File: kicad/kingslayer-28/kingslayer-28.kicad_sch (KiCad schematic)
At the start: 68 parts, among them IC1 STM32F303CCT7, IC2 IS31FL3731-QFLS2-TR, K1 KEYSW, K10 KEYSW, K11 KEYSW, K12 KEYSW, K13 KEYSW, K14 KEYSW, K15 KEYSW, K16 KEYSW, K17 KEYSW, K18 KEYSW, K19 KEYSW, K2 KEYSW, K20 KEYSW, K21 KEYSW, K22 KEYSW, K23 KEYSW, K24 KEYSW, K25 KEYSW, K26 KEYSW, K27 KEYSW, K28 KEYSW, K3 KEYSW, K4 KEYSW, K5 KEYSW, K6 KEYSW, K7 KEYSW, K8 KEYSW, K9 KEYSW, SW1 SW_PUSH, X1 XTAL_GND

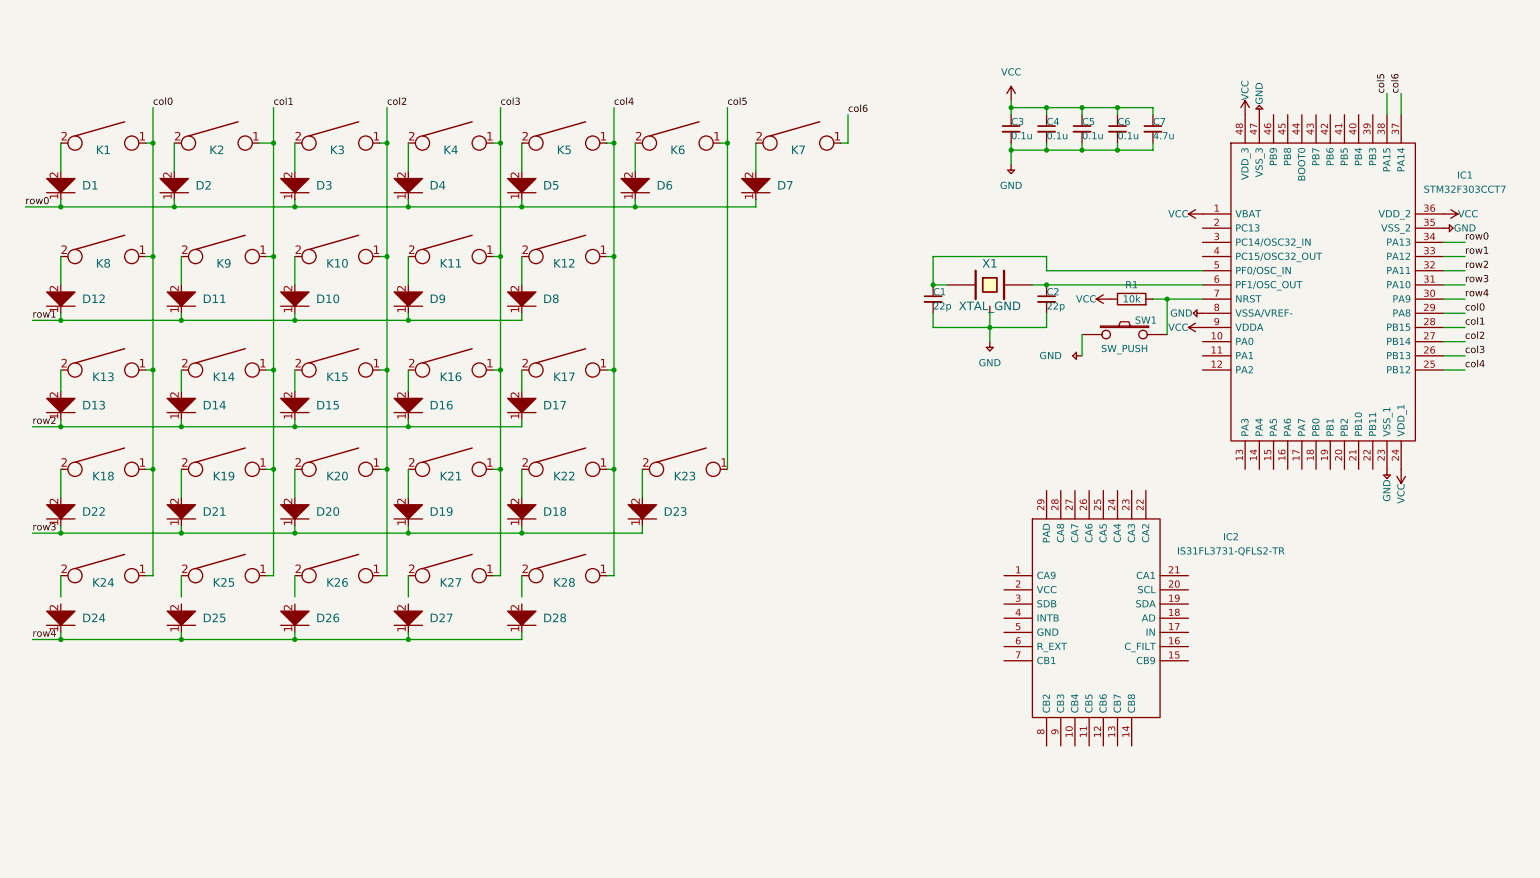
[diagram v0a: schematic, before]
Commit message: tidy up the schematic
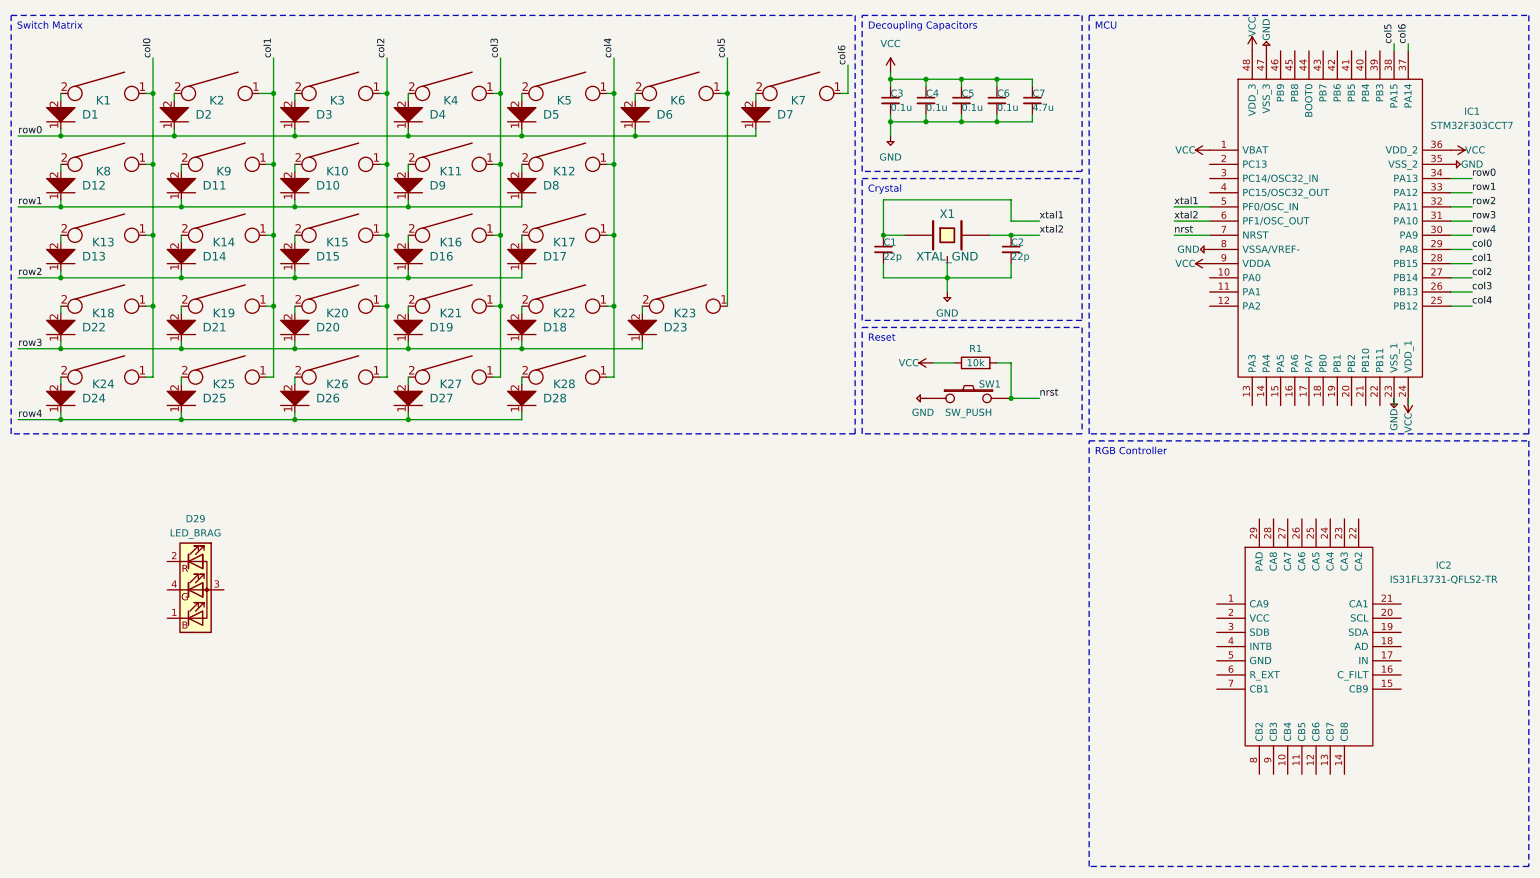
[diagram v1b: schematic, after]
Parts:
- added D29: LED_BRAG, symbol Device:LED_BRAG
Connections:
- net xtal1: now reaches C1.1, IC1.5 (PF0/OSC_IN), X1.1
- net xtal2: now reaches C2.1, IC1.6 (PF1/OSC_OUT), X1.2
- net nrst: now reaches IC1.7 (NRST), R1.2, SW1.2
- net at K26.2: now also D26.2
- net at D28.2: now also K28.2
- net at D24.2: now also K24.2
- net at D25.2: now also K25.2
- net at K27.2: now also D27.2
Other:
- moved on the sheet: C1, C2, C3, C4, C5, C6, C7, D1, D10, D11, D12, D13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
